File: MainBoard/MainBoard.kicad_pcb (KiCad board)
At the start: 4 copper layers, 70 x 70 mm, 25 parts, among them IC1 MAX30102, J1 PV IN, J2 Micro_SD_Card, J3 USB_C_Receptacle, U1 MAX-8C, U2 TPS61201DRC, U3 STM32WL55CCU7, U4 LSM9DS1, U5 FUSB302B01MPX

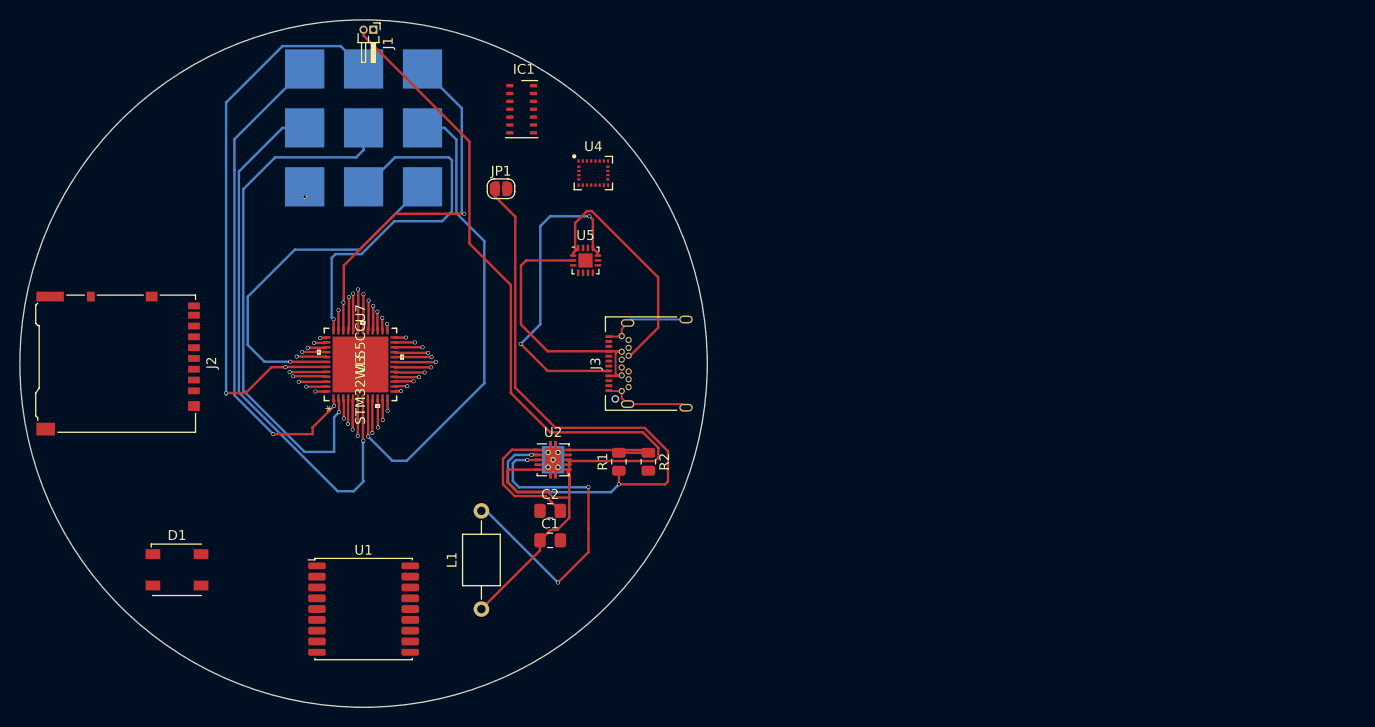
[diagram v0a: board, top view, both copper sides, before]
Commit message: lots of work on PCB
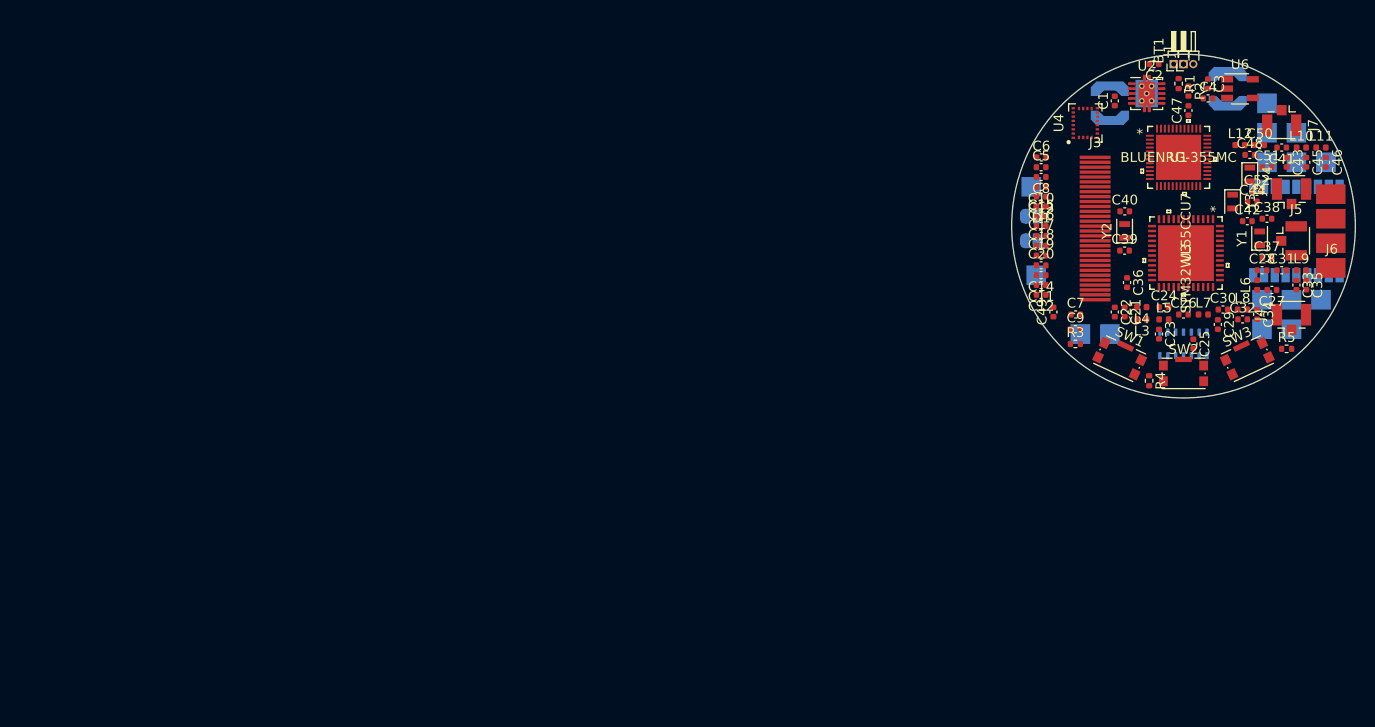
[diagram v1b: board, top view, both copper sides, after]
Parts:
- removed U5: FUSB302B01MPX, Package_DFN_QFN:WQFN-14-1EP_2.5x2.5mm_P0.5mm_EP1.45x1.45mm
- added BT1: Battery_Cell, Connector_PinHeader_1.00mm:PinHeader_1x02_P1.00mm_Horizontal, F.Cu at (133.5, 18.5)
- added C10: 0.1uF, Capacitor_SMD:C_0402_1005Metric, F.Cu at (120.0, 31.0)
- added C11: 0.1uF, Capacitor_SMD:C_0402_1005Metric, F.Cu at (120.0, 41.0)
- added C12: 0.1uF, Capacitor_SMD:C_0402_1005Metric, F.Cu at (120.0, 42.0)
- added C13: 0.1uF, Capacitor_SMD:C_0402_1005Metric, F.Cu at (120.0, 32.0)
- added C14: 2.2uF, Capacitor_SMD:C_0402_1005Metric, F.Cu at (120.0, 40.0)
- added C15: 0.1uF, Capacitor_SMD:C_0402_1005Metric, F.Cu at (120.0, 34.0)
- added C16: 0.1uF, Capacitor_SMD:C_0402_1005Metric, F.Cu at (120.0, 35.0)
- added C17: 0.1uF, Capacitor_SMD:C_0402_1005Metric, F.Cu at (120.0, 36.0)
- added C18: 0.1uF, Capacitor_SMD:C_0402_1005Metric, F.Cu at (120.0, 37.0)
- added C19: 0.1uF, Capacitor_SMD:C_0402_1005Metric, F.Cu at (120.0, 38.0)
- added C20: 0.1uF, Capacitor_SMD:C_0402_1005Metric, F.Cu at (120.0, 39.0)
- added C21: 0.1uF, Capacitor_SMD:C_0402_1005Metric, F.Cu at (128.5, 43.8)
- added C22: 0.1uF, Capacitor_SMD:C_0402_1005Metric, F.Cu at (127.5, 43.8)
- added C23: 0.1uF, Capacitor_SMD:C_0402_1005Metric, F.Cu at (132.0, 46.0)
- added C24: 0.1uF, Capacitor_SMD:C_0402_1005Metric, F.Cu at (132.5, 43.2)
- added C25: 0.1uF, Capacitor_SMD:C_0402_1005Metric, F.Cu at (135.5, 47.0)
- added C26: 0.1uF, Capacitor_SMD:C_0402_1005Metric, F.Cu at (134.5, 44.0)
- added C27: 0.1uF, Capacitor_SMD:C_0402_1005Metric, F.Cu at (143.5, 41.5)
- added C28: 0.1uF, Capacitor_SMD:C_0402_1005Metric, F.Cu at (142.5, 39.5)
- added C29: 0.1uF, Capacitor_SMD:C_0402_1005Metric, F.Cu at (138.0, 45.0)
- added C3: 4.7uF, Capacitor_SMD:C_0402_1005Metric, F.Cu at (137.0, 20.5)
- added C30: 0.1uF, Capacitor_SMD:C_0402_1005Metric, F.Cu at (138.5, 43.5)
- added C31: 0.1uF, Capacitor_SMD:C_0402_1005Metric, F.Cu at (144.5, 39.5)
- added C32: 0.1uF, Capacitor_SMD:C_0402_1005Metric, F.Cu at (140.5, 44.5)
- added C33: 0.1uF, Capacitor_SMD:C_0402_1005Metric, F.Cu at (146.0, 41.0)
- added C34: 0.1uF, Capacitor_SMD:C_0402_1005Metric, F.Cu at (142.0, 44.0)
- added C35: 0.1uF, Capacitor_SMD:C_0402_1005Metric, F.Cu at (147.0, 41.0)
- added C36: _, Capacitor_SMD:C_0402_1005Metric, F.Cu at (128.8, 40.8)
- added C37: _, Capacitor_SMD:C_0402_1005Metric, F.Cu at (143.0, 38.2)
- added C38: _, Capacitor_SMD:C_0402_1005Metric, F.Cu at (143.0, 34.2)
- added C39: _, Capacitor_SMD:C_0402_1005Metric, F.Cu at (128.5, 37.5)
- added C4: 10uF, Capacitor_SMD:C_0402_1005Metric, F.Cu at (137.0, 22.0)
- added C40: _, Capacitor_SMD:C_0402_1005Metric, F.Cu at (128.5, 33.5)
- added C41: _, Capacitor_SMD:C_0402_1005Metric, F.Cu at (144.5, 27.0)
- added C42: _, Capacitor_SMD:C_0402_1005Metric, F.Cu at (141.0, 34.5)
- added C43: _, Capacitor_SMD:C_0402_1005Metric, F.Cu at (145.0, 28.5)
- added C44: _, Capacitor_SMD:C_0402_1005Metric, F.Cu at (141.5, 32.5)
- added C45: _, Capacitor_SMD:C_0402_1005Metric, F.Cu at (147.0, 28.5)
- added C46: _, Capacitor_SMD:C_0402_1005Metric, F.Cu at (149.0, 28.5)
- added C47: _, Capacitor_SMD:C_0402_1005Metric, F.Cu at (135.0, 23.2)
- added C48: _, Capacitor_SMD:C_0402_1005Metric, F.Cu at (141.2, 27.8)
- added C49: _, Capacitor_SMD:C_0402_1005Metric, F.Cu at (121.2, 43.8)
- added C5: 0.1uF, Capacitor_SMD:C_0402_1005Metric, F.Cu at (120.0, 29.0)
- added C50: _, Capacitor_SMD:C_0402_1005Metric, F.Cu at (142.2, 26.8)
- added C51: _, Capacitor_SMD:C_0402_1005Metric, F.Cu at (143.0, 29.0)
- added C52: _, Capacitor_SMD:C_0402_1005Metric, F.Cu at (142.0, 31.5)
- added C6: 1uF, Capacitor_SMD:C_0402_1005Metric, F.Cu at (120.0, 28.0)
- added C7: 4.7uF, Capacitor_SMD:C_0402_1005Metric, F.Cu at (123.5, 44.0)
- added C8: 0.1uF, Capacitor_SMD:C_0402_1005Metric, F.Cu at (120.0, 30.0)
- added C9: 0.1uF, Capacitor_SMD:C_0402_1005Metric, F.Cu at (123.5, 45.5)
- added IC2: TESEO-LIV3F, libs:SON110P970X1010X230-18N, B.Cu at (146.0, 35.5)
- added J4: RX, Connector_Coaxial:U.FL_Hirose_U.FL-R-SMT-1_Vertical, F.Cu at (145.5, 44.5)
- added J5: RX, Connector_Coaxial:U.FL_Hirose_U.FL-R-SMT-1_Vertical, F.Cu at (145.5, 36.5)
- added J6: Conn_01x04, libs:4 Pin SMD Wire, F.Cu at (149.5, 35.5)
- added J7: Conn_Coaxial, Connector_Coaxial:U.FL_Hirose_U.FL-R-SMT-1_Vertical, F.Cu at (144.5, 24.2)
- added JP2: BAT EN, Jumper:SolderJumper-2_P1.3mm_Open_RoundedPad1.0x1.5mm, B.Cu at (119.0, 34.0)
- added L10: _, Inductor_SMD:L_0402_1005Metric, F.Cu at (146.5, 27.0)
- added L11: _, Inductor_SMD:L_0402_1005Metric, F.Cu at (148.5, 27.0)
- added L12: _, Inductor_SMD:L_0402_1005Metric, F.Cu at (140.2, 26.8)
- added L2: 1uH, Inductor_SMD:L_Coilcraft_LPS4018, B.Cu at (139.0, 21.0)
- added L3: 1uH, Inductor_SMD:L_0402_1005Metric, F.Cu at (130.2, 44.5)
- added L4: 1uH, Inductor_SMD:L_0402_1005Metric, F.Cu at (130.2, 43.2)
- added L5: 1uH, Inductor_SMD:L_0402_1005Metric, F.Cu at (132.5, 44.5)
- added L6: 1uH, Inductor_SMD:L_0402_1005Metric, F.Cu at (142.0, 41.0)
- added L7: 1uH, Inductor_SMD:L_0402_1005Metric, F.Cu at (136.5, 44.0)
- added L8: 1uH, Inductor_SMD:L_0402_1005Metric, F.Cu at (140.5, 43.5)
- added L9: 1uH, Inductor_SMD:L_0402_1005Metric, F.Cu at (146.5, 39.5)
- added R3: R_US, Resistor_SMD:R_0402_1005Metric, F.Cu at (123.5, 47.0)
- added R4: R_US, Resistor_SMD:R_0402_1005Metric, F.Cu at (131.0, 50.8)
- added R5: R_US, Resistor_SMD:R_0402_1005Metric, F.Cu at (145.0, 47.5)
- added SW1: SW_DIP_x01, Button_Switch_SMD:SW_Push_1P1T-SH_NO_CK_KMR2xxG, F.Cu at (128.0, 48.5)
- added SW2: SW_DIP_x01, Button_Switch_SMD:SW_Push_1P1T-SH_NO_CK_KMR2xxG, F.Cu at (134.5, 50.0)
- added SW3: SW_DIP_x01, Button_Switch_SMD:SW_Push_1P1T-SH_NO_CK_KMR2xxG, F.Cu at (141.0, 48.5)
- added TP10: GND, TestPoint:TestPoint_Pad_2.0x2.0mm, B.Cu at (143.0, 22.5)
- added TP11: BATT, TestPoint:TestPoint_Pad_2.0x2.0mm, B.Cu at (143.0, 25.5)
- added TP12: RX, TestPoint:TestPoint_Pad_2.0x2.0mm, B.Cu at (145.5, 45.5)
- added TP13: TX, TestPoint:TestPoint_Pad_2.0x2.0mm, B.Cu at (143.0, 28.5)
- added TP14: 3.3V, TestPoint:TestPoint_Pad_2.0x2.0mm, B.Cu at (142.5, 45.5)
- added TP15: BLE RSTN, TestPoint:TestPoint_Pad_2.0x2.0mm, B.Cu at (119.5, 40.0)
- added U6: ADP2108AUJ-3.3, Package_TO_SOT_SMD:TSOT-23-5, F.Cu at (140.2, 21.0)
- added Y1: Crystal, Crystal:Crystal_SMD_2012-2Pin_2.0x1.2mm, F.Cu at (142.2, 36.2)
- added Y2: Crystal, Crystal:Crystal_SMD_2012-2Pin_2.0x1.2mm, F.Cu at (128.5, 35.5)
- added Y3: Crystal, Crystal:Crystal_SMD_2012-2Pin_2.0x1.2mm, F.Cu at (139.5, 32.5)
- added Y4: Crystal, Crystal:Crystal_SMD_2012-2Pin_2.0x1.2mm, F.Cu at (141.2, 29.8)
- C1, C2: footprint Capacitor_SMD:C_0805_2012Metric_Pad1.18x1.45mm_HandSolder -> Capacitor_SMD:C_0402_1005Metric
- D1: value Inolux_IN-PI554FCH -> DIODE; footprint LED_SMD:LED_Inolux_IN-PI554FCH_PLCC4_5.0x5.0mm_P3.2mm -> Diode_SMD:D_0402_1005Metric
- IC1, JP1: moved to B.Cu
- J2: value Micro_SD_Card -> Conn_Coaxial; footprint Connector_Card:microSD_HC_Hirose_DM3AT-SF-PEJM5 -> Connector_Coaxial:U.FL_Hirose_U.FL-R-SMT-1_Vertical
- J3: value USB_C_Receptacle -> Conn_01x30_Female; footprint Connector_USB:USB_C_Receptacle_Amphenol_12401548E4-2A -> libs:waveshare_1.02
- L1: footprint Inductor_THT:L_Axial_L5.0mm_D3.6mm_P10.00mm_Horizontal_Murata_BL01RN1A2A2 -> Inductor_SMD:L_Coilcraft_LPS4018; moved to B.Cu
- R1, R2: footprint Resistor_SMD:R_0805_2012Metric -> Resistor_SMD:R_0402_1005Metric
- TP1: value PWR-REGLP2S -> NRST; footprint TestPoint:TestPoint_Pad_4.0x4.0mm -> TestPoint:TestPoint_Pad_2.0x2.0mm
- TP2, TP4, TP7, TP8, TP9: footprint TestPoint:TestPoint_Pad_4.0x4.0mm -> TestPoint:TestPoint_Pad_2.0x2.0mm
- TP3: value PWR-REGLP1S -> BLE TX; footprint TestPoint:TestPoint_Pad_4.0x4.0mm -> TestPoint:TestPoint_Pad_2.0x2.0mm
- TP5: value RF-NRST -> PA10; footprint TestPoint:TestPoint_Pad_4.0x4.0mm -> TestPoint:TestPoint_Pad_2.0x2.0mm
- TP6: value RF-SMPSRDY -> BLE RX; footprint TestPoint:TestPoint_Pad_4.0x4.0mm -> TestPoint:TestPoint_Pad_2.0x2.0mm
- U1: value MAX-8C -> BLUENRG-355MC; footprint RF_GPS:ublox_MAX -> libs:BLUENRG
- moved J2 120.7 mm to (145.5, 31.7), turned to 90 degrees
- moved TP4 104.4 mm to (149.0, 28.5)
- moved TP9 100.3 mm to (148.5, 42.5)
- moved D1 95.5 mm to (120.0, 33.0), turned to 180 degrees
- moved TP8 95.2 mm to (145.5, 42.5)
- moved TP2 95.0 mm to (146.0, 25.5)
- moved U1 94.9 mm to (134.0, 28.0)
- moved TP1 89.1 mm to (146.0, 28.5)
- moved TP7 86.3 mm to (142.5, 42.5)
- moved U3 84.8 mm to (134.8, 37.8), turned to 270 degrees
- moved J1 82.6 mm to (134.5, 18.5), turned to 90 degrees
- moved L1 82.1 mm to (127.0, 22.5)
- moved TP6 80.4 mm to (124.0, 46.0)
- moved C2 76.5 mm to (131.5, 18.5), turned to 180 degrees
- moved TP5 75.0 mm to (127.0, 46.0)
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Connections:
- D1 pad 1: GND -> Net-(D1-Pad1)
- D1 pad 2: (no net) -> GND
- J2 pad 1: (no net) -> Net-(IC2-Pad11)
- J2 pad 2: (no net) -> GND
- JP1 pad 2: +3V3 -> Net-(BT1-Pad1)
- U1 pad 1: GND -> (no net)
- U1 pad 10: GND -> Net-(TP5-Pad1)
- U1 pad 11: (no net) -> Net-(TP3-Pad1)
- U1 pad 12: GND -> Net-(TP6-Pad1)
- U1 pad 16: SDA -> (no net)
- U1 pad 17: SCL -> (no net)
- U3 pad 10: (no net) -> RX1
- U3 pad 11: (no net) -> +3V3
- U3 pad 12: (no net) -> Net-(J3-Pad5)
- U3 pad 13: (no net) -> SPI1-SCK
- U3 pad 15: (no net) -> Net-(IC2-Pad4)
- U3 pad 16: (no net) -> Net-(IC2-Pad5)
- U3 pad 17: (no net) -> TX
- U3 pad 18: (no net) -> Net-(TP1-Pad1)
- U3 pad 20: (no net) -> RFI_P
- U3 pad 23: (no net) -> RFO_HP
- U3 pad 24: (no net) -> VR_PA
- U3 pad 26: (no net) -> Net-(C38-Pad1)
- U3 pad 27: (no net) -> Net-(C37-Pad1)
- U3 pad 28: (no net) -> +3V3
- U3 pad 3: (no net) -> SPI1-MOSI
- U3 pad 31: Net-(TP6-Pad1) -> (no net)
- U3 pad 32: (no net) -> Net-(R4-Pad1)
- U3 pad 33: (no net) -> RX
- U3 pad 34: Net-(TP5-Pad1) -> Net-(J3-Pad6)
- U3 pad 35: (no net) -> Net-(R3-Pad1)
- U3 pad 38: (no net) -> Net-(R5-Pad1)
- U3 pad 39: (no net) -> Net-(C40-Pad1)
- U3 pad 4: (no net) -> SCL
- U3 pad 40: (no net) -> Net-(C39-Pad1)
- U3 pad 41: (no net) -> Net-(C36-Pad1)
- U3 pad 44: (no net) -> +3V3
- U3 pad 5: (no net) -> SDA
- U3 pad 6: (no net) -> Net-(J3-Pad7)
- U3 pad 7: Net-(TP3-Pad1) -> Net-(J3-Pad8)
- U3 pad 8: Net-(TP1-Pad1) -> Net-(J3-Pad9)
- U3 pad 9: (no net) -> TX1
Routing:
- net Net-(C1-Pad1): track 103.5 -> 0.00 mm
- net (no net): track 96.1 -> 0.00 mm, vias 38 -> 0
- net Net-(JP1-Pad1): track 67.9 -> 0.00 mm, vias 2 -> 0
- net Net-(TP9-Pad1): track 58.6 -> 0.00 mm, vias 2 -> 0
- net Net-(TP3-Pad1): track 56.7 -> 0.00 mm, vias 1 -> 0
- net Net-(TP2-Pad1): track 54.1 -> 0.00 mm, vias 1 -> 0
- net Net-(TP4-Pad1): track 50.2 -> 0.00 mm, vias 2 -> 0
- net Net-(TP1-Pad1): track 49.8 -> 0.00 mm, vias 1 -> 0
- net Net-(TP5-Pad1): track 37.7 -> 0.00 mm, vias 2 -> 0
- net Net-(TP8-Pad1): track 37.2 -> 0.00 mm, vias 1 -> 0
- net Net-(TP7-Pad1): track 36.1 -> 0.00 mm, vias 1 -> 0
- net Net-(L1-Pad2): track 34.4 -> 0.00 mm, vias 3 -> 0
- net Net-(J3-PadA5): track 32.7 -> 0.00 mm, vias 2 -> 0
- net Net-(J3-PadA4): track 27.7 -> 0.00 mm
- net Net-(J3-PadB5): track 24.9 -> 0.00 mm
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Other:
- board size 70 x 70 mm -> 35 x 35 mm

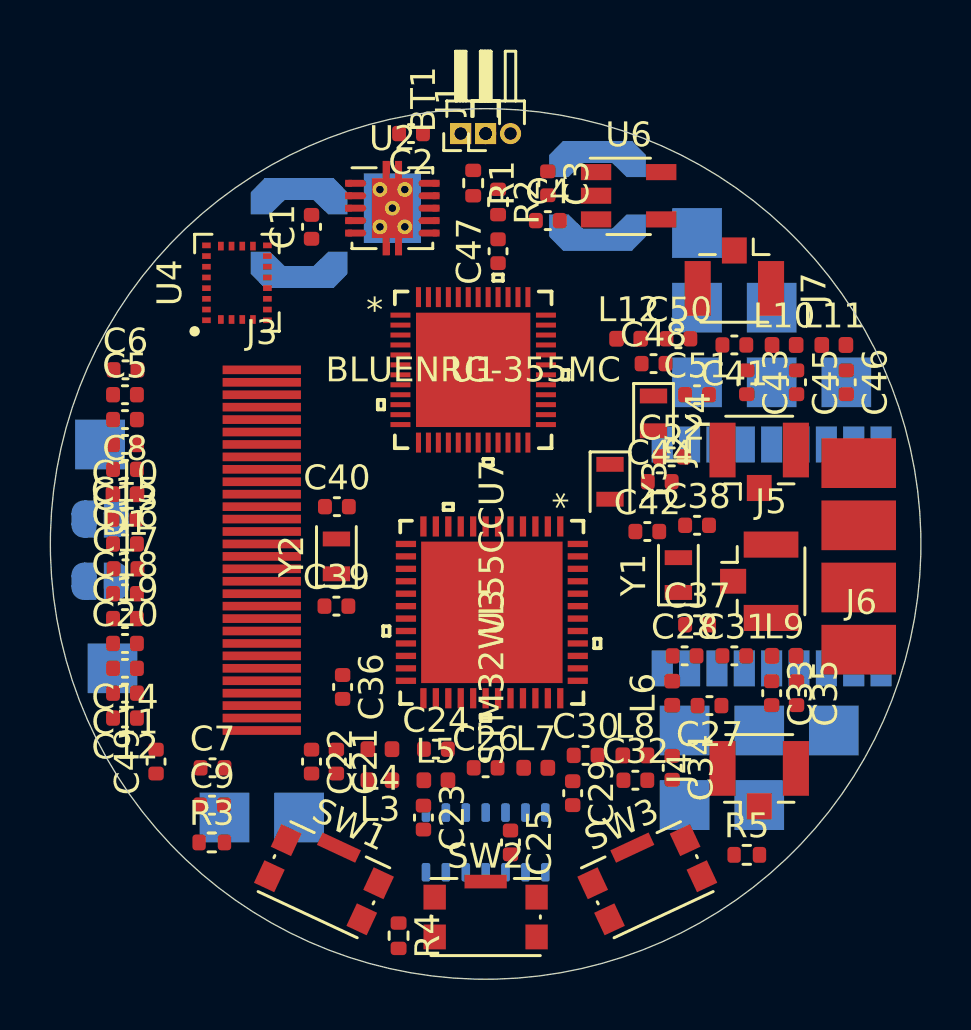
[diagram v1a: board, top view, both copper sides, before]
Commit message: lots of work on PCB
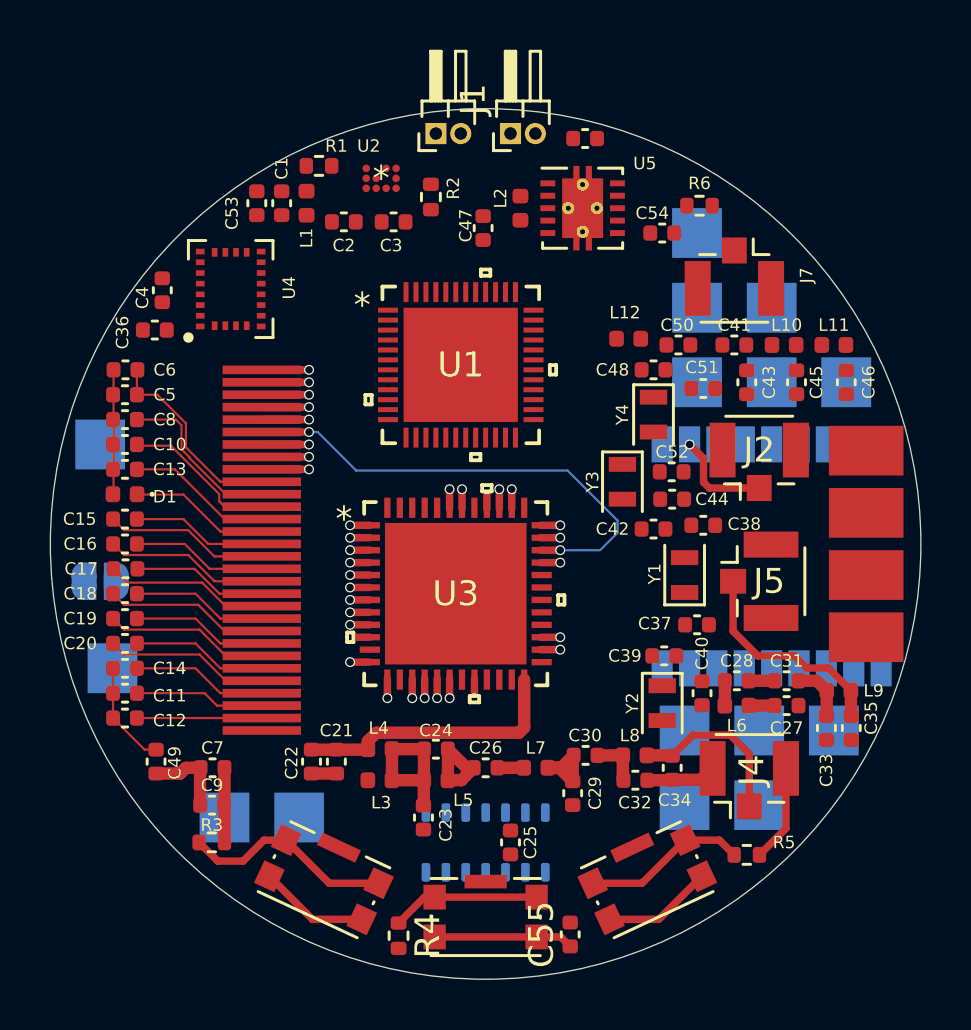
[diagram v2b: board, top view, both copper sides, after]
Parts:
- removed JP2: BAT EN, Jumper:SolderJumper-2_P1.3mm_Open_RoundedPad1.0x1.5mm
- removed U6: ADP2108AUJ-3.3, Package_TO_SOT_SMD:TSOT-23-5
- added C53: 10uF, Capacitor_SMD:C_0402_1005Metric, F.Cu at (125.3, 21.3)
- added C54: 0.1uF, Capacitor_SMD:C_0402_1005Metric, F.Cu at (141.6, 22.5)
- added C55: 10uF, Capacitor_SMD:C_0402_1005Metric, F.Cu at (137.9, 50.7)
- added C56: 10uF, Capacitor_SMD:C_0402_1005Metric, F.Cu at (138.5, 18.7)
- added R6: 100, Resistor_SMD:R_0402_1005Metric, F.Cu at (143.1, 21.4)
- added U5: TPS63001, Package_SON:Texas_DRC0010J_ThermalVias, F.Cu at (138.4, 21.5)
- C1: value 10uF -> 1uF
- C2: value 0.1uF -> 1uF
- C3: value 4.7uF -> 1uF
- C36: value _ -> 100uF
- C4: value 10uF -> 10nF
- L1: value 2.2uH -> INDUCTOR; footprint Inductor_SMD:L_Coilcraft_LPS4018 -> Inductor_SMD:L_0402_1005Metric; moved to F.Cu
- L2: footprint Inductor_SMD:L_Coilcraft_LPS4018 -> Inductor_SMD:L_0402_1005Metric; moved to F.Cu
- R1: value SET R1 -> 5K
- R2: value SET R2 -> R_US
- U2: value TPS61201DRC -> MAX20361AEWC+; footprint Package_SON:Texas_S-PVSON-N10_ThermalVias -> libs:MAX20361AEWC&plus_
- moved C40 16.5 mm to (143.2, 41.0), turned to 270 degrees
- moved C36 16.2 mm to (121.2, 26.4), turned to 0 degrees
- moved C4 15.8 mm to (121.5, 24.8), turned to 90 degrees
- moved Y2 14.4 mm to (141.6, 41.4), turned to 270 degrees
- moved C39 13.3 mm to (141.7, 39.5), turned to 180 degrees
- moved C3 6.39 mm to (130.8, 22.1), turned to 0 degrees
- moved R1 6.24 mm to (127.8, 19.8), turned to 0 degrees
- moved C2 4.46 mm to (128.8, 22.1)
- moved L2 3.14 mm to (135.9, 21.5)
- moved C27 3.10 mm to (146.6, 41.5)
- moved R2 2.71 mm to (132.3, 21.1), turned to 90 degrees
- moved L6 2.65 mm to (144.6, 41.5), turned to 180 degrees
- moved C33 2.61 mm to (148.2, 42.4)
- moved C35 2.61 mm to (149.2, 42.4)
- moved L9 2.61 mm to (148.7, 40.9)
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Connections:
- C1 pad 1: Net-(C1-Pad1) -> (no net)
- C2 pad 1: GND -> Net-(C2-Pad1)
- C2 pad 2: Net-(C2-Pad2) -> GND
- C3 pad 1: Net-(BT1-Pad1) -> Net-(C3-Pad1)
- C3 pad 2: +3V3 -> GND
- C4 pad 1: +3V3 -> Net-(C4-Pad1)
- IC1 pad 10: (no net) -> +3V3
- IC1 pad 9: (no net) -> +3V3
- J1 pad 2: Net-(C1-Pad1) -> Net-(J1-Pad2)
- JP1 pad 1: Net-(JP1-Pad1) -> Net-(C3-Pad1)
- L1 pad 1: Net-(C1-Pad1) -> Net-(J1-Pad2)
- L2 pad 2: +3V3 -> Net-(L2-Pad2)
- R1 pad 1: Net-(JP1-Pad1) -> GND
- R2 pad 1: Net-(R1-Pad2) -> Net-(R2-Pad1)
- R2 pad 2: GND -> Net-(R2-Pad2)
- U3 pad 11: +3V3 -> (no net)
- U3 pad 25: +3V3 -> (no net)
- U3 pad 28: +3V3 -> (no net)
- U3 pad 41: Net-(C36-Pad1) -> (no net)
- U3 pad 44: +3V3 -> (no net)
- U4 pad 13: (no net) -> +3V3
- U4 pad 14: (no net) -> GND
- U4 pad 15: (no net) -> GND
- U4 pad 16: (no net) -> GND
- U4 pad 17: (no net) -> GND
- U4 pad 18: (no net) -> GND
- U4 pad 21: (no net) -> Net-(C4-Pad1)
- U4 pad 24: (no net) -> Net-(C36-Pad1)
- U4 pad 5: (no net) -> GND
- U4 pad 6: (no net) -> GND
- U4 pad 7: (no net) -> +3V3
- U4 pad 8: (no net) -> +3V3
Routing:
- net GND: track 0.00 -> 21.9 mm, vias 0 -> 1
- net +3V3: track 0.00 -> 19.8 mm, vias 0 -> 1
- net Net-(J3-Pad6): track 0.00 -> 19.7 mm, vias 0 -> 2
- net SPI1-SCK: track 0.00 -> 18.5 mm, vias 0 -> 2
- net Net-(J3-Pad5): track 0.00 -> 15.6 mm, vias 0 -> 2
- net SPI1-MOSI: track 0.00 -> 14.0 mm, vias 0 -> 2
- net Net-(J3-Pad8): track 0.00 -> 13.6 mm, vias 0 -> 2
- net Net-(J3-Pad7): track 0.00 -> 13.4 mm, vias 0 -> 2
- net Net-(J3-Pad9): track 0.00 -> 13.3 mm, vias 0 -> 2
- net VR_PA: track 0.00 -> 11.0 mm
- net Net-(R3-Pad1): track 0.00 -> 9.39 mm, vias 0 -> 1
- net Net-(C35-Pad1): track 0.00 -> 8.76 mm
- net Net-(C5-Pad2): track 0.00 -> 8.04 mm
- net Net-(R5-Pad1): track 0.00 -> 7.44 mm, vias 0 -> 1
- net Net-(C34-Pad1): track 0.00 -> 6.89 mm
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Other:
- net class Default: clearance 0.2 -> 0.09; trace_width 0.25 -> 0.09; via_dia 0.8 -> 0.4; via_drill 0.4 -> 0.3
- rule trace_clearance: 0.2 -> 0.09
- rule trace_min: 0.2 -> 0.09
